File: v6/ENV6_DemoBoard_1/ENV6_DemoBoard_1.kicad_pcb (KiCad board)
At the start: 2 copper layers, 83.6 x 65.2 mm, 112 parts, among them J1 Pico Debugger (SWD), J2 Micro_SD_Card, J3 Conn_02x12_Odd_Even, U1 RP2354B, U2 Pi-Radio, U3 W25Q16JVUXIQ, U4 BQ25188, U5 PAC1954x-x4MX, U6 TPSM8310x, U7 PAC1954x-x4MX, U8 PAC1954x-x4MX, Y1 KX7_QRZ

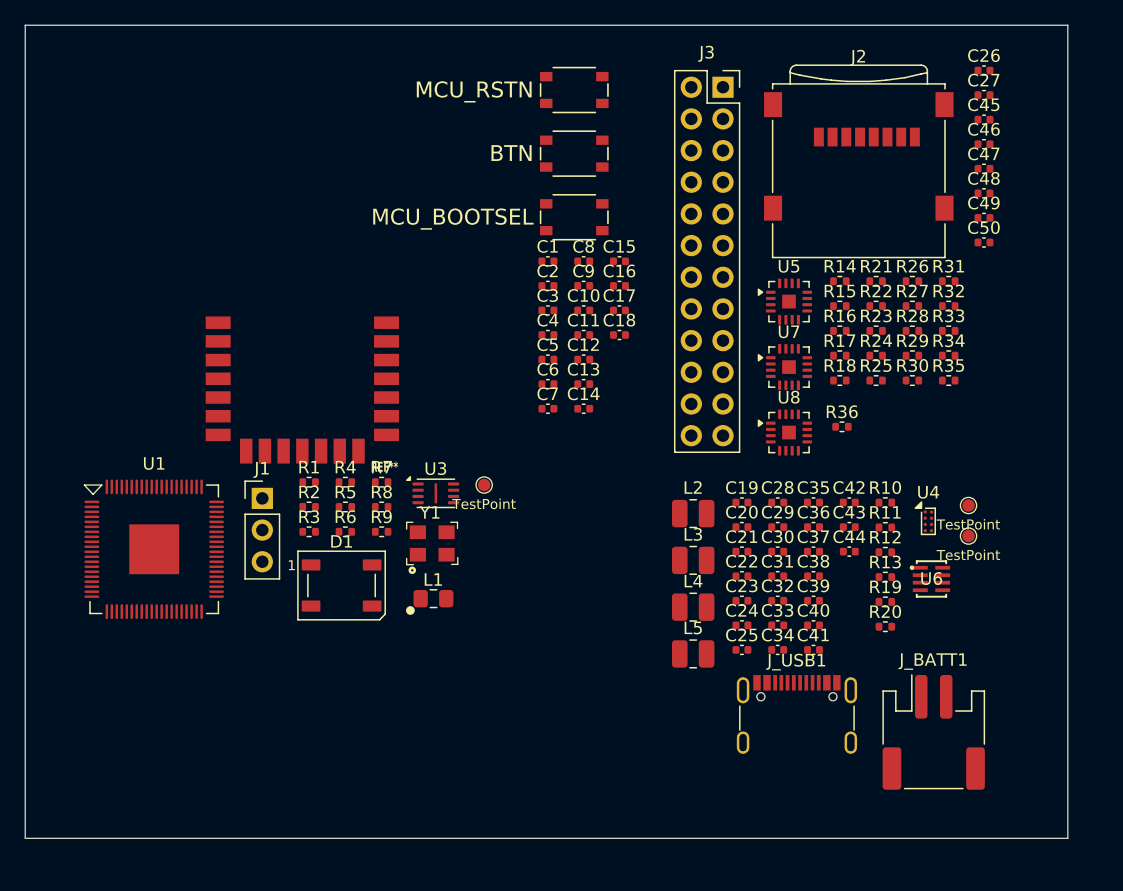
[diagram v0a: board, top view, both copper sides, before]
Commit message: first rev Base Board pcb layout
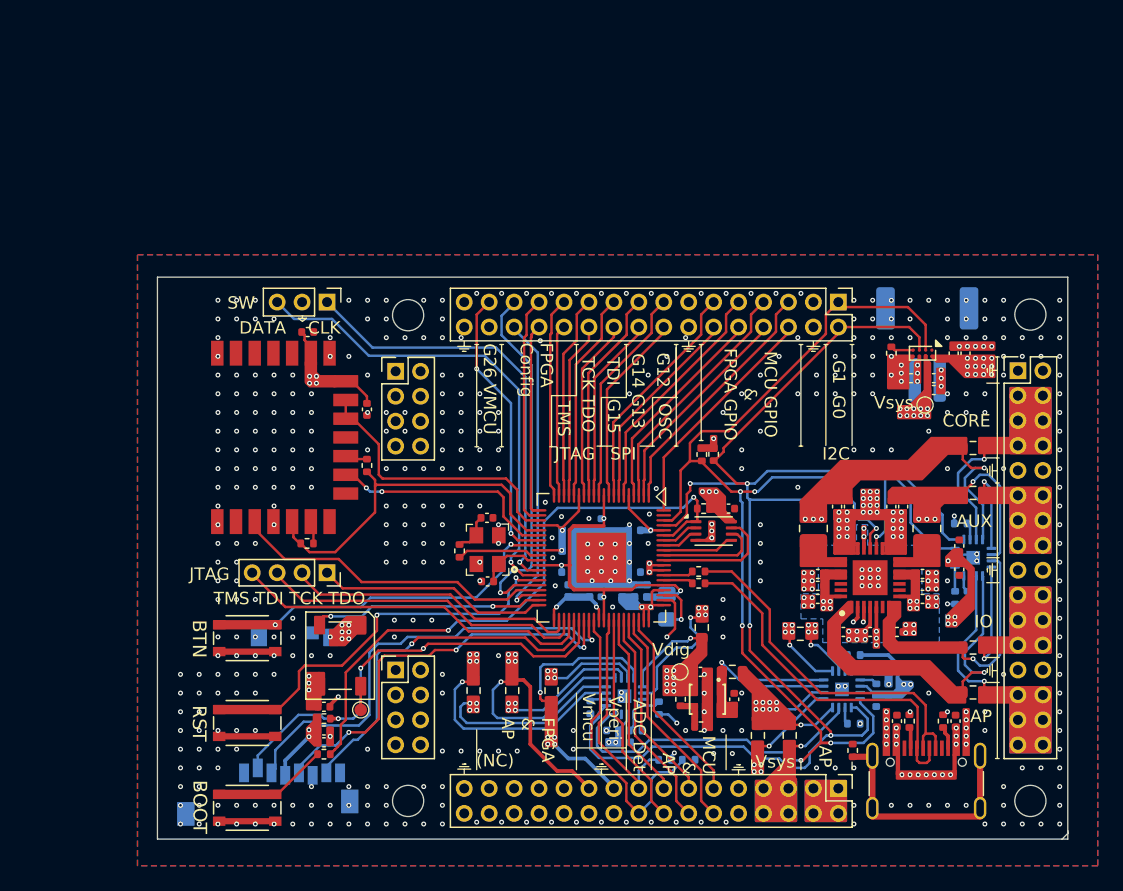
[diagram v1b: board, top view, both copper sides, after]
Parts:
- removed C1, C10, C13, C14, C15, C16, C2, C20, C21, C24, C27, C3, C4, C46, C47, C5, C50, C6, C7, C8, C9: 100n, Capacitor_SMD:C_0402_1005Metric
- removed C11, C12, C19, C22, C23, C25, C26, C28, C29, C30, C31, C32, C33, C34, C35, C36, C37, C38, C39, C40, C41, C42, C43, C44, C45, C48, C49: 10u, Capacitor_SMD:C_0402_1005Metric
- removed C17, C18: 16p, Capacitor_SMD:C_0402_1005Metric
- removed D1: WS2812B, LED_SMD:LED_WS2812B_PLCC4_5.0x5.0mm_P3.2mm
- removed J1: Pico Debugger (SWD), Connector_PinHeader_2.54mm:PinHeader_1x03_P2.54mm_Vertical
- removed J2: Micro_SD_Card, connectors:microSD_HC_Wuerth_693072010801
- removed J3: Conn_02x12_Odd_Even, Connector_PinSocket_2.54mm:PinSocket_2x12_P2.54mm_Vertical
- removed J_BATT1: S2B-PH-SM4-TB, Connector_JST:JST_PH_S2B-PH-SM4-TB_1x02-1MP_P2.00mm_Horizontal
- removed J_USB1: USB-C Receptable (16P), connectors:USB_C_Receptacle_16P
- removed L1: 3µ3, custom_library:L_0805_2012_metric_Alligned_HandSolder
- removed L2, L3, L4, L5: 0.47uH, Inductor_SMD:L_1008_2520Metric
- removed R1, R10, R11, R13, R2: 5k1, Resistor_SMD:R_0402_1005Metric
- removed R12, R15, R22, R28, R30, R6, R7: 10k, Resistor_SMD:R_0402_1005Metric
- removed R14, R16, R21, R23, R24, R25, R29, R31, R32, R33, R36: 0R82, Resistor_SMD:R_0402_1005Metric
- removed R17: 100k, Resistor_SMD:R_0402_1005Metric
- removed R18, R27, R34, R35, R5, R8, R9: 750R, Resistor_SMD:R_0402_1005Metric
- removed R19: 511k, Resistor_SMD:R_0402_1005Metric
- removed R20: 91k, Resistor_SMD:R_0402_1005Metric
- removed R26: 0R1, Resistor_SMD:R_0402_1005Metric
- removed R3, R4: 27R, Resistor_SMD:R_0402_1005Metric
- removed S1: MCU_RSTN, connectors:TACTILE-SWITCH
- removed S2: BTN, connectors:TACTILE-SWITCH
- removed S3: MCU_BOOTSEL, connectors:TACTILE-SWITCH
- removed TP1, TP2, TP3: TestPoint, custom_library:TestPoint_Pad_D1.0mm
- removed U1: RP2354B, custom_library:QFN-80_EP_10x10_Pitch0.4mm
- removed U2: Pi-Radio, mcu_rpi_pico:RPi-Radio-Module
- removed U3: W25Q16JVUXIQ, custom_library:USON-8-1EP_3x2mm_P0.5mm_EP0.2x1.6mm
- removed U4: BQ25188, Package_BGA:Texas_DSBGA-8_0.9x1.9mm_Layout2x4_P0.5mm
- removed U5, U7, U8: PAC1954x-x4MX, Package_DFN_QFN:VQFN-16-1EP_3x3mm_P0.5mm_EP1.1x1.1mm
- removed U6: TPSM8310x, custom_library:MICROSIP8_SIU_TEX
- removed Y1: KX7_QRZ, custom_library:KX-7
- added C201: 10u, Capacitor_SMD:C_0402_1005Metric, B.Cu at (162.1, 120.1)
- added C202: 100n, Capacitor_SMD:C_0402_1005Metric, B.Cu at (161.1, 119.2)
- added C203: 10u, Capacitor_SMD:C_0402_1005Metric, F.Cu at (188.9, 106.2)
- added C204: 100n, Capacitor_SMD:C_0402_1005Metric, F.Cu at (188.9, 104.3)
- added C205: 10u, Capacitor_SMD:C_0402_1005Metric, B.Cu at (182.2, 116.8)
- added C206: 100n, Capacitor_SMD:C_0402_1005Metric, B.Cu at (183.2, 115.8)
- added C207: 100n, Capacitor_SMD:C_0402_1005Metric, F.Cu at (137.9, 120.1)
- added C208: 10u, Capacitor_SMD:C_0402_1005Metric, F.Cu at (137.9, 119.2)
- added C301: 100n, Capacitor_SMD:C_0402_1005Metric, F.Cu at (188.6, 118.4)
- added C302: 10u, Capacitor_SMD:C_0402_1005Metric, F.Cu at (183.9, 118.4)
- added C303: 10u, Capacitor_SMD:C_0402_1005Metric, F.Cu at (188.4, 88.9)
- added C304: 100n, Capacitor_SMD:C_0402_1005Metric, F.Cu at (189.4, 88.9)
- added C305: 10u, Capacitor_SMD:C_0402_1005Metric, F.Cu at (186.8, 90.9)
- added C306: 100n, Capacitor_SMD:C_0402_1005Metric, F.Cu at (186.8, 91.8)
- added C307: 10u, Capacitor_SMD:C_0402_1005Metric, F.Cu at (185.0, 90.9)
- added C308: 10u, Capacitor_SMD:C_0402_1005Metric, F.Cu at (177.6, 106.6)
- added C309: 10u, Capacitor_SMD:C_0402_1005Metric, F.Cu at (177.6, 107.5)
- added C310: 10u, Capacitor_SMD:C_0402_1005Metric, F.Cu at (185.9, 106.6)
- added C311: 10u, Capacitor_SMD:C_0402_1005Metric, F.Cu at (185.9, 107.5)
- added C312: 10u, Capacitor_SMD:C_0402_1005Metric, F.Cu at (177.6, 108.6)
- added C313: 10u, Capacitor_SMD:C_0402_1005Metric, F.Cu at (185.9, 108.6)
- added C314: 10u, Capacitor_SMD:C_0402_1005Metric, F.Cu at (181.8, 111.2)
- added C315: 10u, Capacitor_SMD:C_0402_1005Metric, F.Cu at (179.6, 111.2)
- added C316: 10u, Capacitor_SMD:C_0402_1005Metric, F.Cu at (183.9, 111.2)
- added C317: 10u, Capacitor_SMD:C_0402_1005Metric, F.Cu at (179.1, 101.2)
- added C318: 10u, Capacitor_SMD:C_0402_1005Metric, F.Cu at (184.4, 101.2)
- added C319: 10u, Capacitor_SMD:C_0402_1005Metric, F.Cu at (180.1, 101.2)
- added C320: 10u, Capacitor_SMD:C_0402_1005Metric, F.Cu at (183.4, 101.2)
- added C321: 10u, Capacitor_SMD:C_0402_1005Metric, F.Cu at (170.8, 116.7)
- added C322: 10u, Capacitor_SMD:C_0402_1005Metric, F.Cu at (168.1, 114.5)
- added C401: 100n, Capacitor_SMD:C_0402_1005Metric, B.Cu at (160.2, 102.7)
- added C402: 100n, Capacitor_SMD:C_0402_1005Metric, B.Cu at (157.5, 106.5)
- added C403: 100n, Capacitor_SMD:C_0402_1005Metric, B.Cu at (160.2, 108.0)
- added C404: 100n, Capacitor_SMD:C_0402_1005Metric, B.Cu at (162.8, 103.1)
- added C405: 100n, Capacitor_SMD:C_0402_1005Metric, B.Cu at (162.8, 106.5)
- added C406: 100n, Capacitor_SMD:C_0402_1005Metric, B.Cu at (157.6, 103.1)
- added C407: 100n, Capacitor_SMD:C_0402_1005Metric, B.Cu at (157.6, 104.8)
- added C408: 100n, Capacitor_SMD:C_0402_1005Metric, B.Cu at (157.6, 108.0)
- added C409: 100n, Capacitor_SMD:C_0402_1005Metric, B.Cu at (161.9, 108.0)
- added C410: 100n, Capacitor_SMD:C_0402_1005Metric, B.Cu at (159.2, 108.0)
- added C411: 10u, Capacitor_SMD:C_0402_1005Metric, B.Cu at (162.8, 108.0)
- added C412: 10u, Capacitor_SMD:C_0402_1005Metric, B.Cu at (163.8, 108.0)
- added C413: 100n, Capacitor_SMD:C_0402_1005Metric, F.Cu at (137.9, 117.2)
- added C414: 100n, Capacitor_SMD:C_0402_1005Metric, F.Cu at (170.4, 101.4)
- added C415: 100n, Capacitor_SMD:C_0402_1005Metric, F.Cu at (141.4, 93.4)
- added C416: 100n, Capacitor_SMD:C_0402_1005Metric, F.Cu at (136.7, 87.2)
- added C417: 16p, Capacitor_SMD:C_0402_1005Metric, F.Cu at (151.0, 102.1)
- added C418: 16p, Capacitor_SMD:C_0402_1005Metric, F.Cu at (151.1, 107.2)
- added D401: WS2812B, LED_SMD:LED_WS2812B_PLCC4_5.0x5.0mm_P3.2mm, F.Cu at (139.2, 113.2)
- added G***: LOGO, logos:logo_ude_5x5, B.Cu at (178.2, 91.8)
- added H501: MountingHole, MountingHole:MountingHole_2.5mm, F.Cu at (144.7, 85.8)
- added H502: MountingHole, MountingHole:MountingHole_2.5mm, F.Cu at (194.6, 85.8)
- added H503: MountingHole, MountingHole:MountingHole_2.5mm, F.Cu at (144.7, 124.8)
- added H504: MountingHole, MountingHole:MountingHole_2.5mm, F.Cu at (194.6, 124.8)
- added IC301: LP873300RHDTQ1, custom_library:QFN50P500X500X80-29N, F.Cu at (181.8, 106.9)
- added J201: MEM2052-00-195-00-A, ui_stuff:MEM20520019500A, B.Cu at (133.4, 118.9)
- added J401: Pico Debugger (SWD), Connector_PinHeader_2.00mm:PinHeader_1x03_P2.00mm_Vertical, F.Cu at (138.2, 84.8)
- added J402: Conn_01x04_Pin, Connector_PinSocket_2.00mm:PinSocket_1x04_P2.00mm_Vertical, F.Cu at (138.2, 106.5)
- added J501: Conn_02x16_Odd_Even, Connector_PinHeader_2.00mm:PinHeader_2x16_P2.00mm_Vertical, F.Cu at (164.2, 85.8)
- added J502: Conn_02x04_Odd_Even, Connector_PinHeader_2.00mm:PinHeader_2x04_P2.00mm_Vertical, F.Cu at (144.7, 93.3)
- added J503: Conn_02x16_Odd_Even, Connector_PinHeader_2.00mm:PinHeader_2x16_P2.00mm_Vertical, F.Cu at (194.6, 105.3)
- added J504: Conn_02x04_Odd_Even, Connector_PinHeader_2.00mm:PinHeader_2x04_P2.00mm_Vertical, F.Cu at (144.7, 117.3)
- added J505: Conn_02x16_Odd_Even, Connector_PinHeader_2.00mm:PinHeader_2x16_P2.00mm_Vertical, F.Cu at (164.2, 124.8)
- added J_BATT301: S2B-PH-SM4-TB, Connector_JST:JST_PH_S2B-PH-SM4-TB_1x02-1MP_P2.00mm_Horizontal, B.Cu at (186.3, 88.2)
- added J_USB301: USB-C Receptable (16P), connectors:USB_C_Receptacle_16P, F.Cu at (186.2, 124.3)
- added L301: 0.47uH, Inductor_SMD:L_1008_2520Metric, F.Cu at (177.2, 103.0)
- added L302: 0.47uH, Inductor_SMD:L_1008_2520Metric, F.Cu at (186.3, 103.0)
- added L401: 3µ3, custom_library:L_0805_2012_metric_Alligned_HandSolder, B.Cu at (165.4, 109.2)
- added NT301: NetTie_2, NetTie:NetTie-2_SMD_Pad0.5mm, B.Cu at (177.5, 104.5)
- added R201: 0R82, Resistor_SMD:R_0603_1608Metric, F.Cu at (156.2, 116.0)
- added R202: 0R82, Resistor_SMD:R_0603_1608Metric, F.Cu at (168.2, 110.9)
- added R203: 0R82, Resistor_SMD:R_0603_1608Metric, F.Cu at (149.9, 116.0)
- added R204: 0R82, Resistor_SMD:R_0603_1608Metric, F.Cu at (153.1, 116.0)
- added R205: 0R1, Resistor_SMD:R_0402_1005Metric, B.Cu at (159.3, 117.3)
- added R206: 750R, Resistor_SMD:R_0402_1005Metric, B.Cu at (162.9, 119.2)
- added R207: 10k, Resistor_SMD:R_0402_1005Metric, B.Cu at (164.8, 117.3)
- added R208: 0R82, Resistor_SMD:R_0603_1608Metric, F.Cu at (190.0, 112.5)
- added R209: 0R82, Resistor_SMD:R_0603_1608Metric, F.Cu at (190.0, 116.1)
- added R210: 0R82, Resistor_SMD:R_0603_1608Metric, F.Cu at (190.0, 96.5)
- added R211: 0R82, Resistor_SMD:R_0603_1608Metric, F.Cu at (190.0, 100.1)
- added R212: 750R, Resistor_SMD:R_0402_1005Metric, B.Cu at (189.0, 102.5)
- added R213: 750R, Resistor_SMD:R_0402_1005Metric, B.Cu at (188.6, 108.5)
- added R214: 10k, Resistor_SMD:R_0402_1005Metric, B.Cu at (189.6, 108.5)
- added R215: 0R82, Resistor_SMD:R_0603_1608Metric, F.Cu at (172.8, 119.5)
- added R216: 0R82, Resistor_SMD:R_0603_1608Metric, F.Cu at (170.7, 114.5)
- added R217: 0R82, Resistor_SMD:R_0603_1608Metric, F.Cu at (176.2, 111.4)
- added R218: 0R82, Resistor_SMD:R_0603_1608Metric, F.Cu at (175.3, 119.5)
- added R219: 100k, Resistor_SMD:R_0402_1005Metric, B.Cu at (180.4, 118.6)
- added R220: 750R, Resistor_SMD:R_0402_1005Metric, B.Cu at (182.2, 114.9)
- added R221: 10k, Resistor_SMD:R_0402_1005Metric, B.Cu at (180.4, 113.1)
- added R222: 10k, Resistor_SMD:R_0402_1005Metric, F.Cu at (137.9, 118.2)
- added R301: 5k1, Resistor_SMD:R_0402_1005Metric, F.Cu at (184.9, 118.4)
- added R302: 5k1, Resistor_SMD:R_0402_1005Metric, F.Cu at (187.6, 118.4)
- added R303: 5k1, Resistor_SMD:R_0402_1005Metric, F.Cu at (180.3, 120.8)
- added R304: 10k, Resistor_SMD:R_0402_1005Metric, F.Cu at (183.4, 88.9)
- added R305: 511k, Resistor_SMD:R_0402_1005Metric, F.Cu at (166.5, 116.7)
- added R306: 91k, Resistor_SMD:R_0402_1005Metric, F.Cu at (168.2, 118.8)
- added R401: 5k1, Resistor_SMD:R_0402_1005Metric, F.Cu at (169.2, 97.0)
- added R402: 5k1, Resistor_SMD:R_0402_1005Metric, F.Cu at (168.2, 97.0)
- added R403: 27R, Resistor_SMD:R_0402_1005Metric, F.Cu at (168.0, 106.4)
- added R404: 27R, Resistor_SMD:R_0402_1005Metric, F.Cu at (168.0, 107.3)
- added R405: 750R, Resistor_SMD:R_0402_1005Metric, F.Cu at (136.6, 104.2)
- added R406: 10k, Resistor_SMD:R_0402_1005Metric, F.Cu at (141.4, 97.9)
- added R407: 10k, Resistor_SMD:R_0402_1005Metric, F.Cu at (168.4, 101.4)
- added R408: 750R, Resistor_SMD:R_0402_1005Metric, F.Cu at (137.9, 121.0)
- added R409: 750R, Resistor_SMD:R_0402_1005Metric, F.Cu at (148.8, 104.8)
- added R410: 10k, Resistor_SMD:R_0402_1005Metric, B.Cu at (167.2, 121.5)
- added R411: 10k, Resistor_SMD:R_0402_1005Metric, B.Cu at (165.3, 121.5)
- added S401: RST, connectors:TACTILE-SWITCH, F.Cu at (131.8, 118.5)
- added S402: BTN, connectors:TACTILE-SWITCH, F.Cu at (131.8, 111.8)
- added S403: BOOT, connectors:TACTILE-SWITCH, F.Cu at (131.8, 125.3)
- added TP301: TestPoint, custom_library:TestPoint_Pad_D1.0mm, F.Cu at (186.2, 93.0)
- added TP302: TestPoint, custom_library:TestPoint_Pad_D1.0mm, F.Cu at (166.5, 114.5)
- added TP401: TestPoint, custom_library:TestPoint_Pad_D1.0mm, F.Cu at (140.9, 117.5)
- added U201: PAC1954x-x4MX, Package_DFN_QFN:VQFN-16-1EP_3x3mm_P0.5mm_EP1.1x1.1mm, B.Cu at (162.1, 116.4)
- added U202: PAC1954x-x4MX, Package_DFN_QFN:VQFN-16-1EP_3x3mm_P0.5mm_EP1.1x1.1mm, B.Cu at (190.0, 105.3)
- added U203: PAC1954x-x4MX, Package_DFN_QFN:VQFN-16-1EP_3x3mm_P0.5mm_EP1.1x1.1mm, B.Cu at (179.5, 115.8)
- added U301: BQ25188, Package_BGA:Texas_DSBGA-8_0.9x1.9mm_Layout2x4_P0.5mm, F.Cu at (185.9, 88.9)
- added U302: TPSM8310x, custom_library:MICROSIP8_SIU_TEX, F.Cu at (168.7, 116.7)
- added U401: RP2354B, custom_library:QFN-80_EP_10x10_Pitch0.4mm, F.Cu at (160.2, 105.3)
- added U402: Pi-Radio, mcu_rpi_pico:RPi-Radio-Module, F.Cu at (131.9, 95.7)
- added U403: W25Q16JVUXIQ, custom_library:USON-8-1EP_3x2mm_P0.5mm_EP0.2x1.6mm, F.Cu at (169.2, 103.2)
- added Y401: KX7_QRZ, custom_library:KX-7, F.Cu at (151.0, 104.7)
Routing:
- net GP0/I2C0_SDA: track 0.00 -> 125.1 mm, vias 0 -> 5
- net GP1/I2C0_SCL: track 0.00 -> 121.9 mm, vias 0 -> 6
- net VDDD_MCU: track 0.00 -> 53.5 mm, vias 0 -> 15
- net Net-(U401-QSPI_SS): track 0.00 -> 48.8 mm, vias 0 -> 2
- net VDDD_PERI: track 0.00 -> 40.3 mm, vias 0 -> 17
- net VDIG_OUT: track 0.00 -> 39.3 mm, vias 0 -> 21
- net Net-(J401-SDATA): track 0.00 -> 39.1 mm, vias 0 -> 1
- net GP39/SPI0_TX: track 0.00 -> 36.7 mm, vias 0 -> 1
- net GP37/SPI0_CS: track 0.00 -> 36.0 mm, vias 0 -> 3
- net Net-(J401-SCLK): track 0.00 -> 35.3 mm, vias 0 -> 1
- net GP38/SPI0_SCK: track 0.00 -> 33.1 mm, vias 0 -> 3
- net CFG_Extra: track 0.00 -> 30.1 mm, vias 0 -> 1
- net GND: track 0.00 -> 30.1 mm, vias 0 -> 497
- net GP36/SPI0_RX: track 0.00 -> 30.1 mm, vias 0 -> 1
- net /MCU/MCU_JTAG_TMS: track 0.00 -> 29.4 mm
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- added copper zone on In2.Cu, net /Power/USB_VCC
- added copper zone on B.Cu, net AGND
- added copper zone on B.Cu, net GND
- added copper zone on F.Cu, net GND
- added copper zone on In1.Cu, net GND
- added copper zone on In2.Cu, net GND
- added copper zone on In2.Cu, net VDDD_FLASH
- added copper zone on In2.Cu, net VDDD_MCU
- added copper zone on In2.Cu, net VDDD_PERI
- added copper zone on In2.Cu, net VDDD_RADIO
- added copper zone on In2.Cu, net VDIG_OUT
- added copper zone on In2.Cu, net VFPGA_IN
- added copper zone on In2.Cu, net VPERI_IN
- added copper zone on In2.Cu, net VSYS_IN
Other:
- board size 83.6 x 65.2 mm -> 73 x 45.1 mm
- copper layers 2 -> 4
- board text added: "(NC)"
- board text added: "ADC Det"
- board text added: "AP"
- board text added: "AUX"
- board text added: "CORE"
- board text added: "DATA CLK"
- board text added: "FPGA & AP"
- board text added: "FPGA Config"
- board text added: "G1 G0"
- board text added: "G12"
- board text added: "G14 G13"
- board text added: "G15"
- board text added: "G26 VMCU"
- board text added: "I2C"
- board text added: "IO"
- board text added: "JTAG"
- board text added: "MCU & AP"
- board text added: "MCU GPIO & FPGA GPIO"
- board text added: "OSC"
- board text added: "SPI"
- board text added: "SW"
- board text added: "TCK TDO"
- board text added: "TDI"
- board text added: "TMS"
- board text added: "TMS TDI TCK TDO"
- board text added: "Vdig"
- board text added: "Vmcu"
- board text added: "Vperi"
- board text added: "Vsys"
- board text added: "elasticAI.hardware ENV6 Base Board 1v0 (c) 2026"
